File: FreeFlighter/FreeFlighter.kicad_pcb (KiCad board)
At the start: 2 copper layers, 41.7 x 20.7 mm, 16 parts

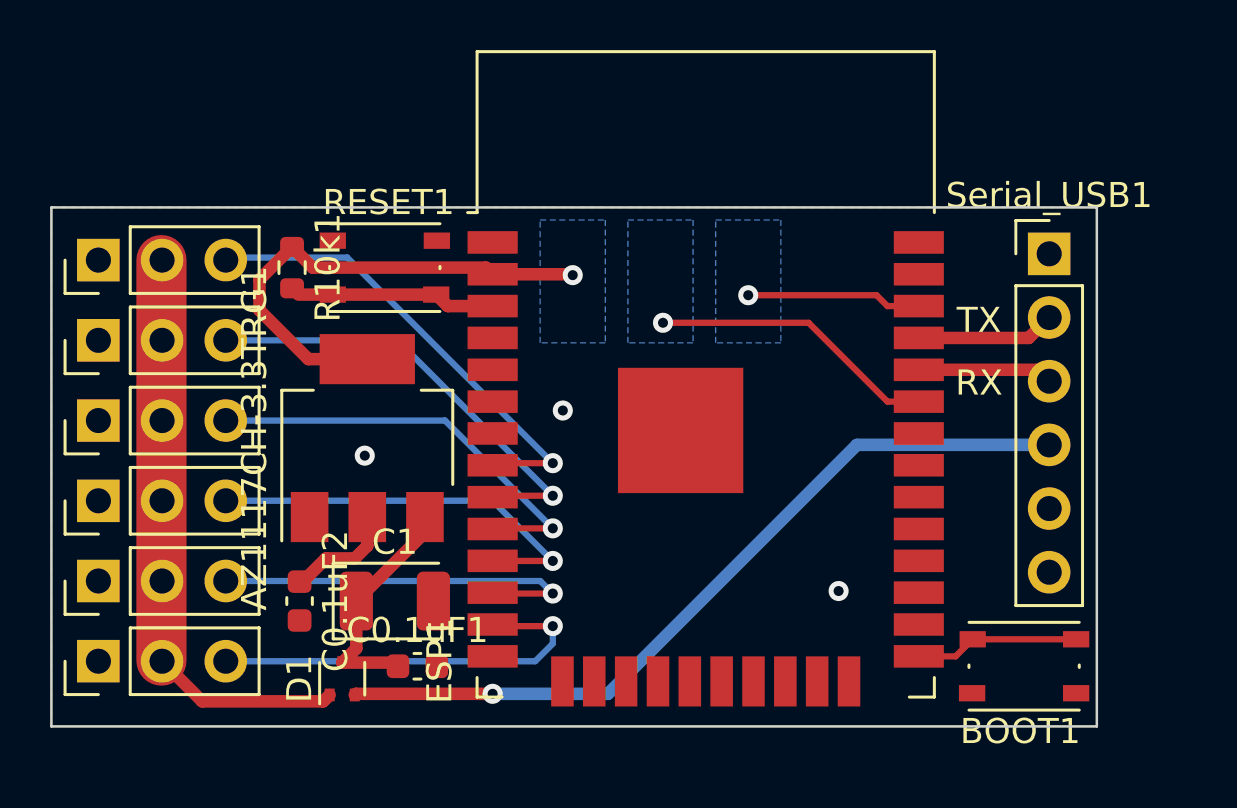
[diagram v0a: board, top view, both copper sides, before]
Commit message: BOM
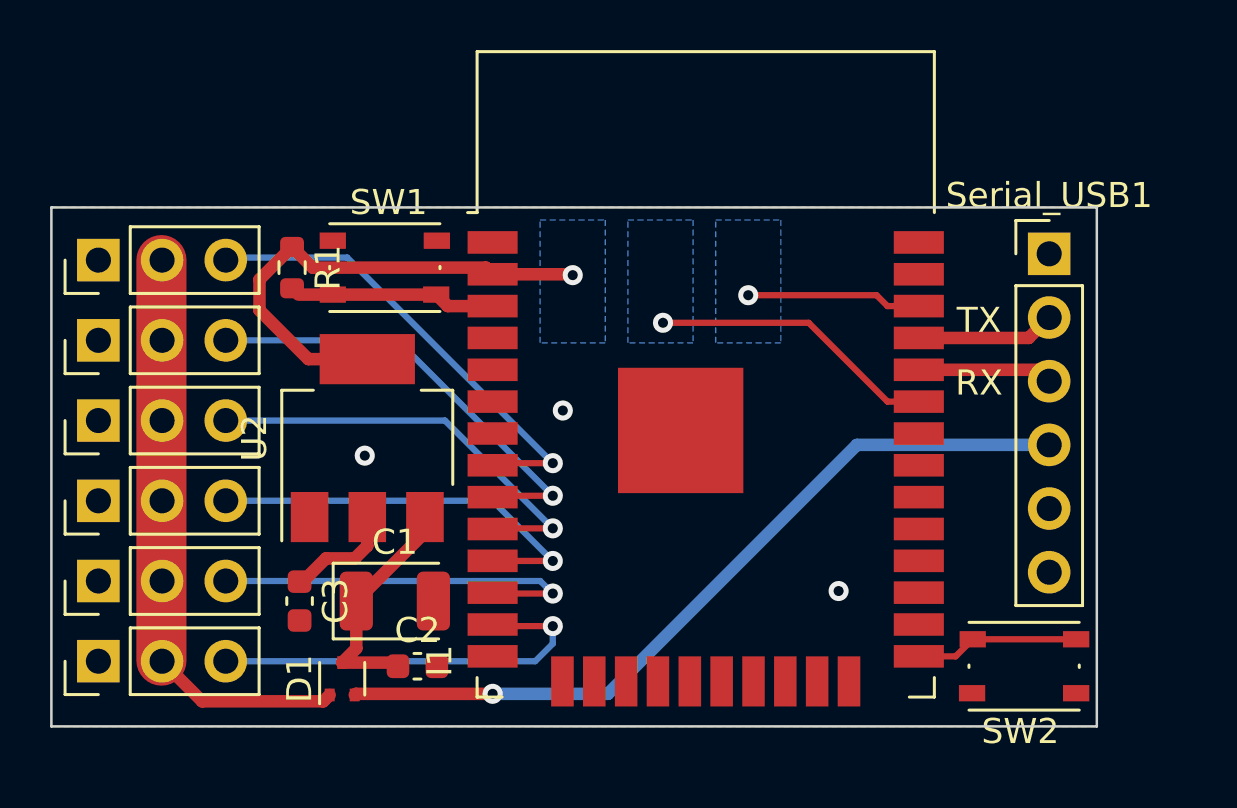
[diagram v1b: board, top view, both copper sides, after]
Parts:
- C1: value C_Polarized -> TAJB226M010R
- C2: renamed from C0.1uF1; value C -> GCM188L81H104K57
- C3: renamed from C0.1uF2; value C -> GCM188L81H104K57
- ESC1, PWM1, PWM2, PWM3, PWM4, RECIV1: value Conn_01x03 -> PH-1x40SG
- I1: renamed from ESP1; value ESP32-WROOM-32 -> ESP32-WROOM-32E
- R1: renamed from R10k1; value R -> RG1608N-102-B-T5
- SW1: renamed from RESET1; value SW_DIP_x01 -> SKRPABE010
- SW2: renamed from BOOT1; value SW_DIP_x01 -> SKRPABE010
- Serial_USB1: value Conn_01x06 -> PH-1x40SG
- U2: renamed from AZ1117CH-3.3TRG1; value LM317_SOT-223 -> AZ1117CH-3.3TRG1
